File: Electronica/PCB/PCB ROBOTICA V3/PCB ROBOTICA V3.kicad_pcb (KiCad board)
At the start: 2 copper layers, 79.2 x 139 mm, 17 parts, among them J1 Ultrasonico 1, J2 Screw_Terminal_01x02, J3 Ultrasonico 2, J4 Ultrasonico 3, J5 Conn_02x05_Counter_Clockwise, J6 Screw_Terminal_01x02

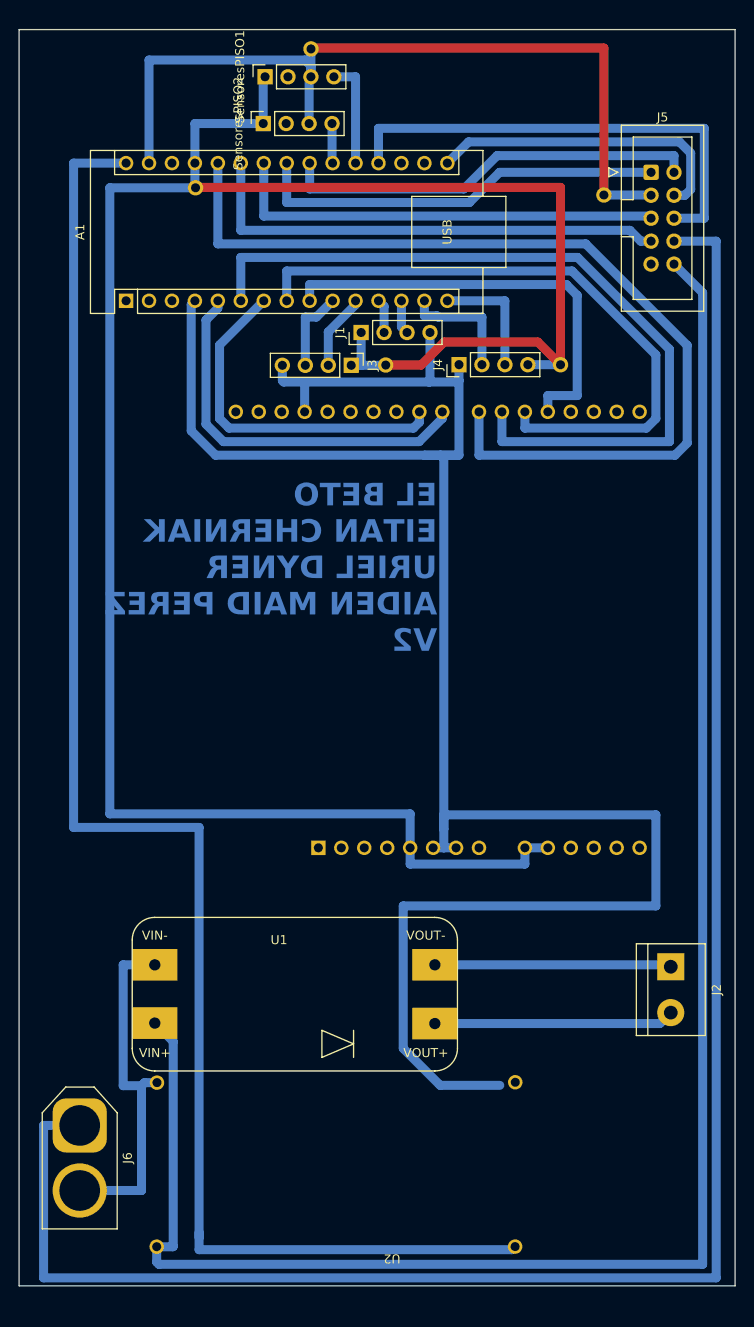
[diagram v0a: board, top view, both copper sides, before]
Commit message: Pcb terminada
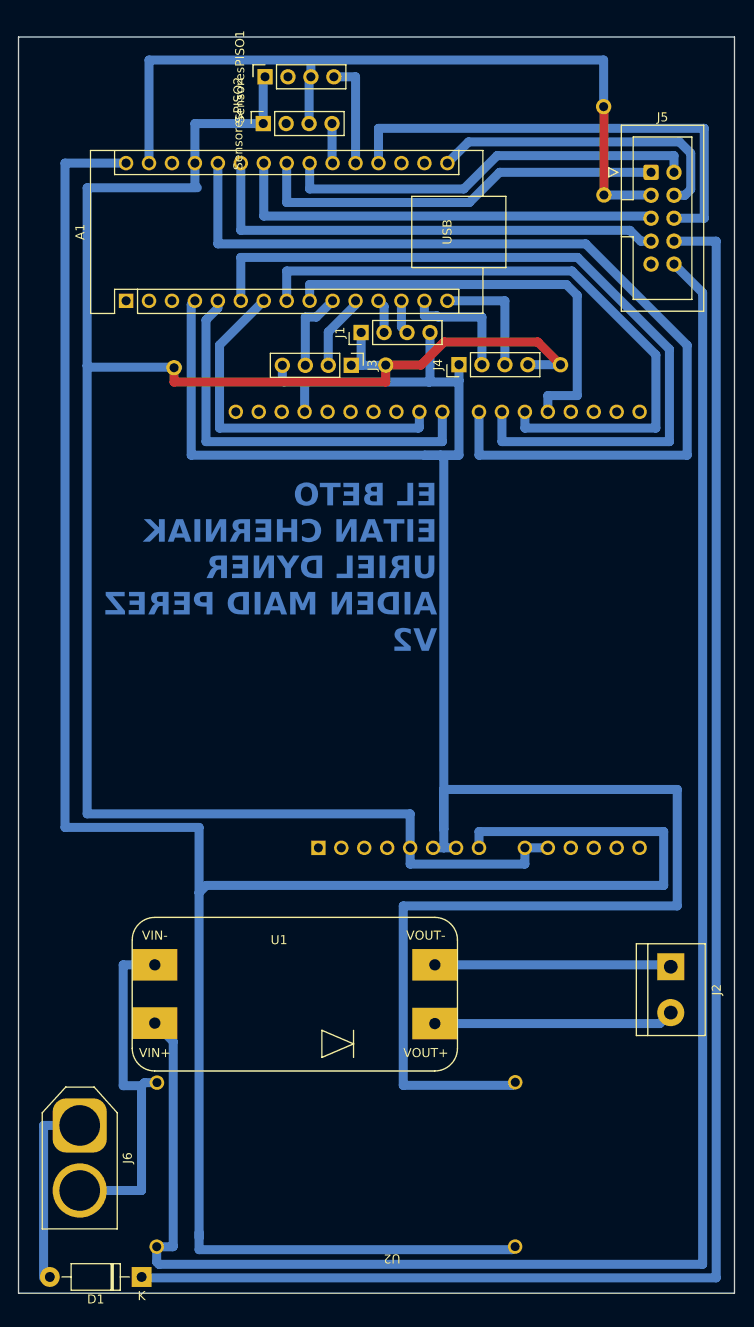
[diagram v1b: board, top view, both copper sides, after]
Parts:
- added D1: 1N4007, Diode_THT:D_DO-41_SOD81_P10.16mm_Horizontal, F.Cu at (127.4, 157.5)
- moved ? 33.0 mm to (178.6, 28.0)
- moved ? 20.1 mm to (131.0, 56.9)
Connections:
- A2 pad 8: unconnected-(A2-VIN-Pad8) -> VIN
- J6 pad 1: SALIDA V BOTONES -> Net-(D1-A)
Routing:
- net VIN: track 175.7 -> 257.6 mm
- net SALIDA V BOTONES: track 214.7 -> 183.1 mm
- net Net-(D1-A): track 0.00 -> 20.9 mm
- net +5V: track 248.0 -> 230.0 mm
- net GND: track 319.1 -> 330.7 mm
- net AIN2 MONSTER SHIELD: track 43.0 -> 45.6 mm
- net BIN 2 MONSTER SHIELD: track 39.0 -> 40.0 mm
- net AIN1 MONSTER SHIELD: track 104.8 -> 105.5 mm
- net PWM A MONSTER SHIELD: track 71.8 -> 72.4 mm
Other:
- board size 79.2 x 139 mm -> 79.2 x 139.1 mm
